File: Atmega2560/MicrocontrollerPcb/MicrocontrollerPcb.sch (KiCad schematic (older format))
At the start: 49 parts, among them J1 Conn_02x12_Odd_Even, U1 ATmega2560-16AU

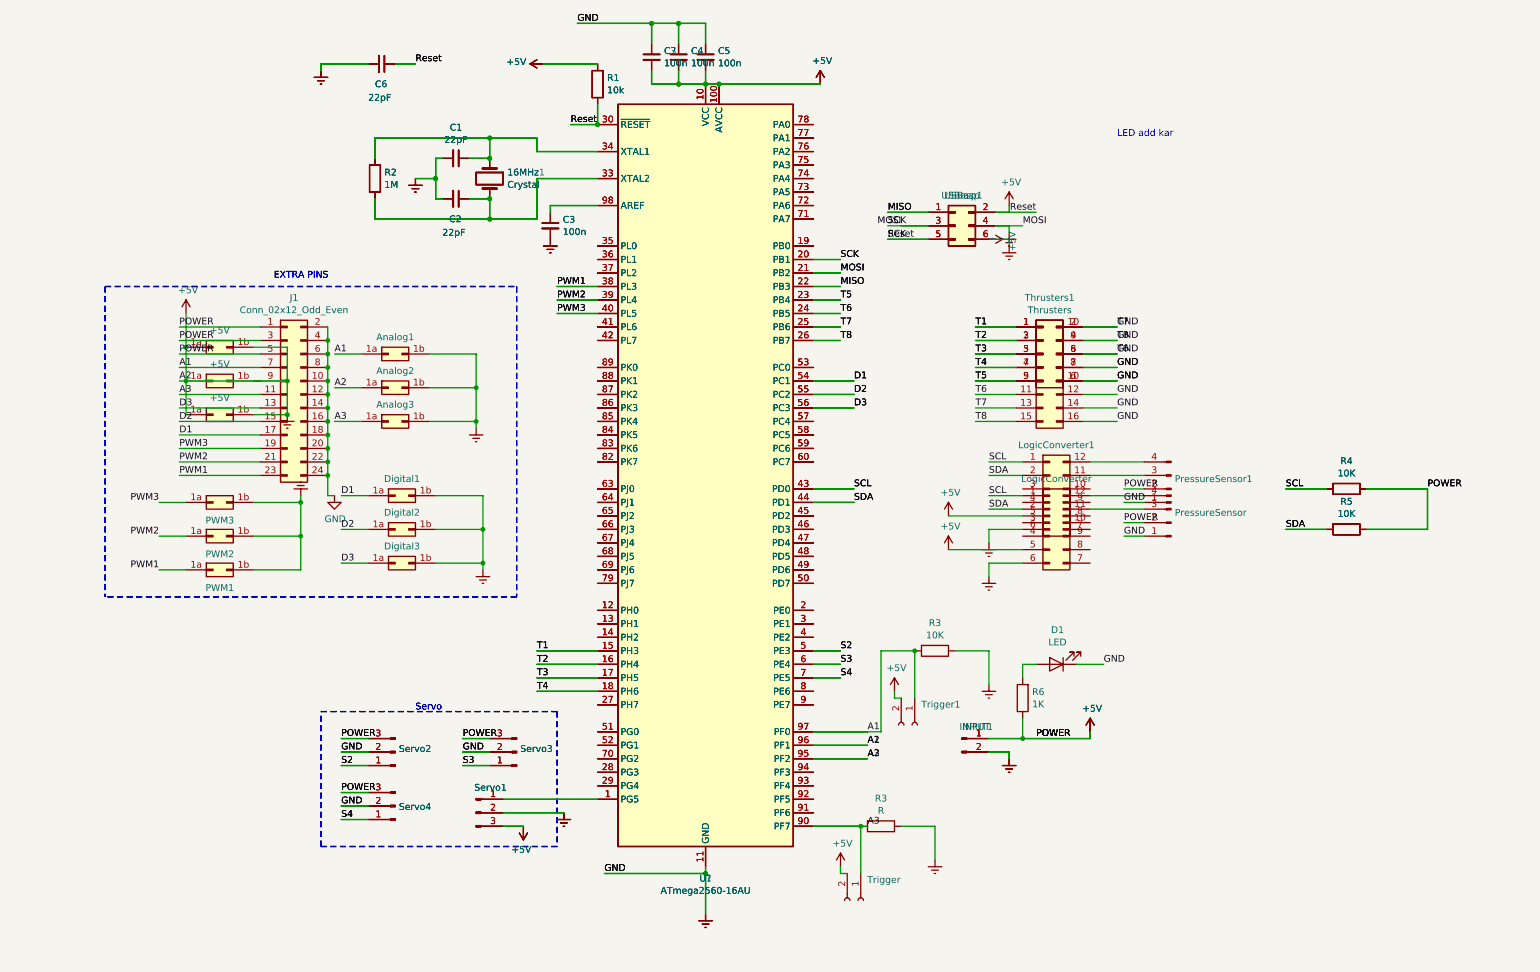
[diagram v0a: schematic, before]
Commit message: self
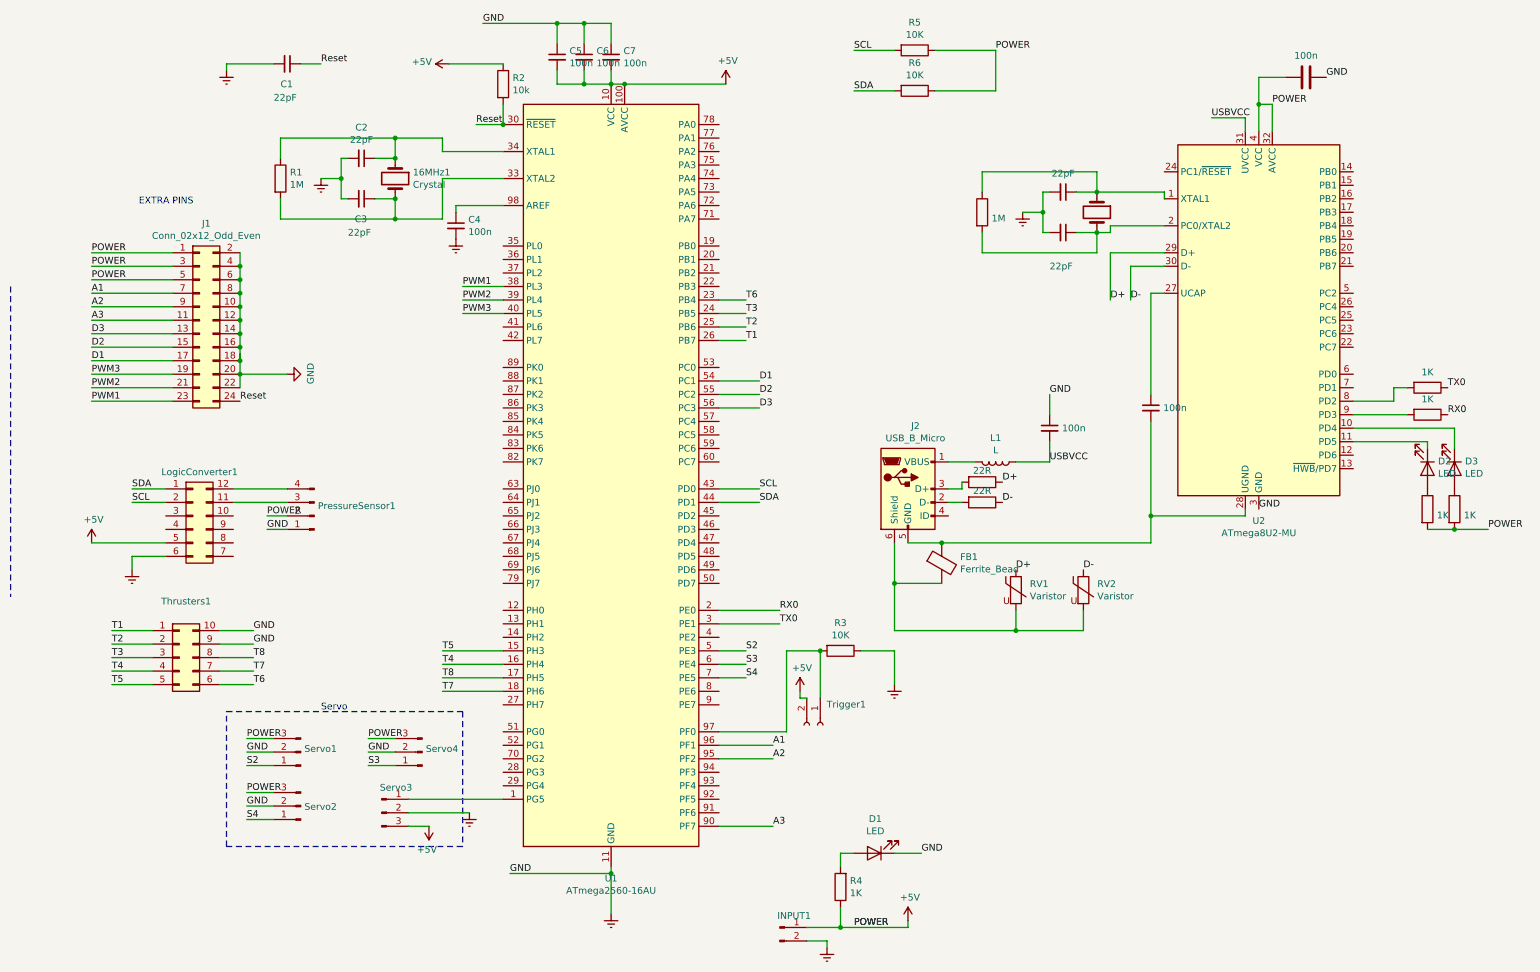
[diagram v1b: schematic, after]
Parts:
- removed +5V (x3), Analog1, Analog2, Analog3, Digital1, Digital2, Digital3, PWM1, PWM2, PWM3: Conn_02x01_Row_Letter_Last, symbol Connector_Generic:Conn_02x01_Row_Letter_Last
- removed 16MHz: Crystal, symbol Device:Crystal
- removed C3 (x2): 100n, symbol Device:C_Small
- removed INPUT: Conn_01x02_Male, symbol Connector:Conn_01x02_Male
- removed LogicConverter: Conn_02x06_Counter_Clockwise, symbol Connector_Generic:Conn_02x06_Counter_Clockwise
- removed PressureSensor: Conn_01x04_Male, symbol Connector:Conn_01x04_Male
- removed R3: R, symbol Device:R
- removed R3: 10K, Resistor_SMD:R_0402_1005Metric, symbol Device:R
- removed R4: 10K, symbol Device:R
- removed Thrusters: Conn_02x08_Odd_Even, symbol Connector_Generic:Conn_02x08_Odd_Even
- removed Trigger: Conn_01x02_Female, symbol Connector:Conn_01x02_Female
- removed U?: ATmega2560-16AU, Package_QFP:TQFP-100_14x14mm_P0.5mm, symbol MCU_Microchip_ATmega:ATmega2560-16AU
- removed USBasp: Conn_02x03_Odd_Even, symbol Connector_Generic:Conn_02x03_Odd_Even
- removed USBasp1: Conn_02x03_Odd_Even, Connector_PinHeader_2.54mm:PinHeader_2x03_P2.54mm_Vertical, symbol Connector_Generic:Conn_02x03_Odd_Even
- added 16MHz2: Crystal, Crystal:Crystal_HC49-U_Vertical, symbol Device:Crystal
- added C10, C3, C9: 22pF, Capacitor_SMD:C_0805_2012Metric_Pad1.15x1.40mm_HandSolder, symbol Device:C_Small
- added C11, C8: 100n, Capacitor_SMD:C_0603_1608Metric_Pad1.05x0.95mm_HandSolder, symbol Device:C_Small
- added C12: 100n, Capacitor_SMD:C_0603_1608Metric_Pad1.05x0.95mm_HandSolder, symbol Device:C
- added D2, D3: LED, LED_SMD:LED_1206_3216Metric, symbol Device:LED
- added FB1: Ferrite_Bead, Resistor_SMD:R_0805_2012Metric, symbol Device:Ferrite_Bead
- added J2: USB_B_Micro, Connector_USB:USB_Micro-B_Amphenol_10103594-0001LF_Horizontal, symbol Connector:USB_B_Micro
- added L1: L, Inductor_SMD:L_1812_4532Metric_Pad1.30x3.40mm_HandSolder, symbol Device:L
- added R10, R11, R12, R13: 1K, Resistor_SMD:R_1206_3216Metric_Pad1.42x1.75mm_HandSolder, symbol Device:R
- added R3, R6: 10K, Resistor_SMD:R_0402_1005Metric, symbol Device:R
- added R7: 1M, Resistor_SMD:R_0402_1005Metric, symbol Device:R
- added R8, R9: 22R, Resistor_SMD:R_0603_1608Metric_Pad1.05x0.95mm_HandSolder, symbol Device:R
- added RV1, RV2: Varistor, Resistor_SMD:R_0603_1608Metric_Pad1.05x0.95mm_HandSolder, symbol Device:Varistor
- added U2: ATmega8U2-MU, Package_DFN_QFN:QFN-32-1EP_5x5mm_P0.5mm_EP3.1x3.1mm, symbol MCU_Microchip_ATmega:ATmega8U2-MU
- C1, C2: footprint (none) -> Capacitor_SMD:C_0805_2012Metric_Pad1.15x1.40mm_HandSolder
- C4, C5: footprint (none) -> Capacitor_SMD:C_0603_1608Metric_Pad1.05x0.95mm_HandSolder
- C6: value 22pF -> 100n; footprint (none) -> Capacitor_SMD:C_0603_1608Metric_Pad1.05x0.95mm_HandSolder
- R1: value 10k -> 1M; footprint (none) -> Resistor_SMD:R_0402_1005Metric
- R2: value 1M -> 10k; footprint (none) -> Resistor_SMD:R_0402_1005Metric
- R5: footprint (none) -> Resistor_SMD:R_0402_1005Metric
- Servo1, Servo2, Servo3, Servo4: footprint (none) -> Molex_Connector:01x03
- renumbered R6 to R4
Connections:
- net +5V: now also R2.1, C12.2, R12.2, R13.2, R6.1, U2.32 (AVCC), U2.4 (VCC); no longer C1.2, C2.2, C4.1, C4.2, C5.1, C6.1, C7.1, D1.1 (K), INPUT1.2 (Pin_2), J1.10 (Pin_10), J1.11 (Pin_11), J1.12 (Pin_12), J1.14 (Pin_14), J1.16 (Pin_16), J1.18 (Pin_18), J1.2 (Pin_2), J1.20 (Pin_20), J1.22 (Pin_22), J1.24 (Pin_24), J1.4 (Pin_4), J1.6 (Pin_6), J1.7 (Pin_7), J1.8 (Pin_8), J1.9 (Pin_9), LogicConverter1.6 (Pin_6), PressureSensor1.1 (Pin_1), R1.1, R1.2, Servo1.2 (Pin_2), Servo2.2 (Pin_2), Servo3.2 (Pin_2), Servo4.2 (Pin_2), Thrusters1.10 (Pin_10), Thrusters1.6 (Pin_6), Thrusters1.7 (Pin_7), Thrusters1.8 (Pin_8), Thrusters1.9 (Pin_9), Trigger1.1 (Pin_1), U1.11 (GND), U1.20 (PB1), U1.21 (PB2), U1.24 (PB5), U1.25 (PB6), U1.26 (PB7), U1.30 (~RESET), U1.32 (GND), U1.62 (GND), U1.81 (GND), U1.90 (PF7), U1.95 (PF2), U1.96 (PF1), U1.97 (PF0), U1.99 (GND)
- net S2: now also Servo1.1 (Pin_1); no longer Servo2.1 (Pin_1)
- net S3: now also Servo4.1 (Pin_1); no longer Servo3.1 (Pin_1)
- net S4: now also Servo2.1 (Pin_1); no longer Servo4.1 (Pin_1)
- net SCL: now also LogicConverter1.2 (Pin_2), R5.2; no longer LogicConverter1.1 (Pin_1)
- net SDA: now also LogicConverter1.1 (Pin_1), R6.2; no longer LogicConverter1.2 (Pin_2), R5.2
- net T1: now also U1.26 (PB7); no longer U1.15 (PH3)
- net T2: now also U1.25 (PB6); no longer U1.16 (PH4)
- net T3: now also U1.24 (PB5); no longer U1.17 (PH5)
- net T4: now also U1.16 (PH4); no longer U1.18 (PH6)
- net T5: now also U1.15 (PH3); no longer U1.23 (PB4)
- net at 16MHz1.1, U1.34 (XTAL1): now also C2.1, R1.1; no longer C1.1, R2.1
- net at 16MHz1.2, U1.33 (XTAL2): now also R1.2, C3.1; no longer C2.1, R2.2
- net at U1.98 (AREF): now also C4.1
- net at U1.1 (PG5): now also Servo3.1 (Pin_1); no longer Servo1.1 (Pin_1)
- net RX0: now reaches U1.2 (PE0)
- net RX0: now also R11.1
- net TX0: now reaches U1.3 (PE1)
- net TX0: now also R10.1
- net MISO: no longer names the net of U1.22 (PB3)
- new net: R3.2, Trigger1.1 (Pin_1), U1.97 (PF0)
- new net: 16MHz2.1, C9.1, R7.1, U2.1 (XTAL1)
- new net: D3.1 (K), U2.10 (PD4)
- new net: D2.1 (K), U2.11 (PD5)
- new net: 16MHz2.2, C10.1, R7.2, U2.2 (PC0/XTAL2)
- new net: C11.1, U2.27 (UCAP)
- new net: C11.2, FB1.1, J2.5 (GND), U2.28 (UGND)
- new net: R10.2, U2.8 (PD2)
- new net: R11.2, U2.9 (PD3)
- new net: D2.2 (A), R12.1
- new net: D3.2 (A), R13.1
- new net: J2.1 (VBUS), L1.2
- new net: J2.2 (D-), R9.2
- new net: J2.3 (D+), R8.2
- new net: FB1.2, J2.6 (Shield), RV1.2, RV2.2
- new net A1: J1.7 (Pin_7), U1.96 (PF1)
- new net A2: J1.9 (Pin_9), U1.95 (PF2)
- new net A3: J1.11 (Pin_11), U1.90 (PF7)
- new net D+: R8.1, RV1.1, U2.29 (D+)
- new net D-: R9.1, RV2.1, U2.30 (D-)
- new net Earth: C1.2, C10.2, C12.1, C2.2, C3.2, C4.2, C5.1, C6.1, C7.1, C8.1, C9.2, D1.1 (K), INPUT1.2 (Pin_2), J1.10 (Pin_10), J1.12 (Pin_12), J1.14 (Pin_14), J1.16 (Pin_16), J1.18 (Pin_18), J1.2 (Pin_2), J1.20 (Pin_20), J1.22 (Pin_22), J1.4 (Pin_4), J1.6 (Pin_6), J1.8 (Pin_8), LogicConverter1.6 (Pin_6), PressureSensor1.1 (Pin_1), R3.1, Servo1.2 (Pin_2), Servo2.2 (Pin_2), Servo3.2 (Pin_2), Servo4.2 (Pin_2), Thrusters1.10 (Pin_10), Thrusters1.9 (Pin_9), U1.11 (GND), U1.32 (GND), U1.62 (GND), U1.81 (GND), U1.99 (GND), U2.3 (GND), U2.33 (GND)
- new net Reset: C1.1, J1.24 (Pin_24), R2.2, U1.30 (~RESET)
- new net T6: Thrusters1.6 (Pin_6), U1.23 (PB4)
- new net T7: Thrusters1.7 (Pin_7), U1.18 (PH6)
- new net T8: Thrusters1.8 (Pin_8), U1.17 (PH5)
- new net USBVCC: C8.2, L1.1, U2.31 (UVCC)
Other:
- note removed: "LED add kar\n"
- moved on the sheet: 16MHz1, C1, C2, C3, C4, C5, C6, C7, D1, INPUT1, J1, LogicConverter1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
